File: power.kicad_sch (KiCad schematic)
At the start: 25 parts, among them U1 ECP5U_12_CABGA256, U2 TLV62569DBV, U3 TLV62569DBV, U4 TLV62569DBV

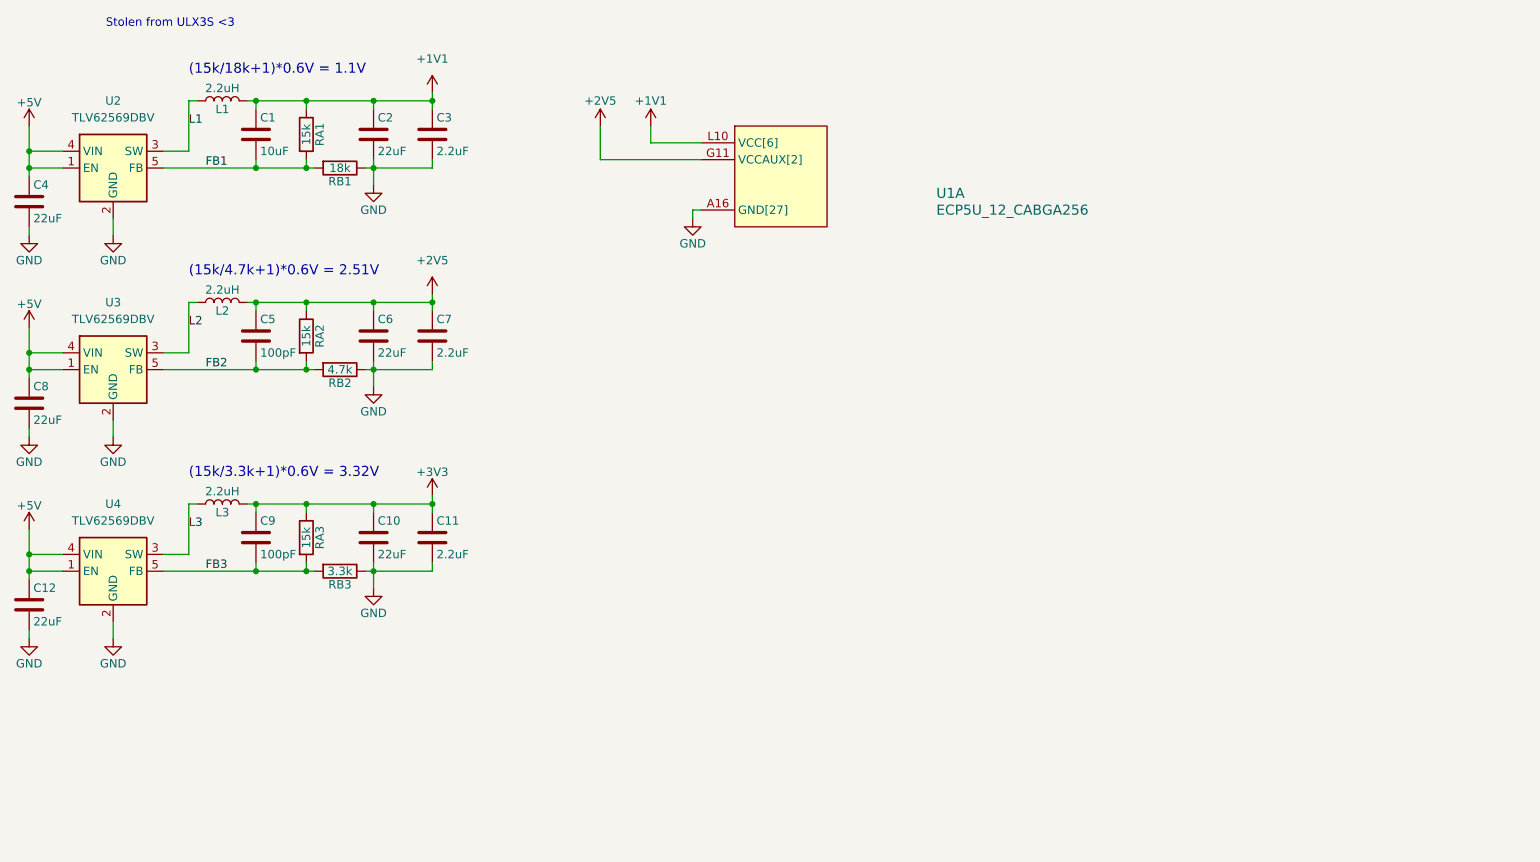
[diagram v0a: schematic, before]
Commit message: Stash
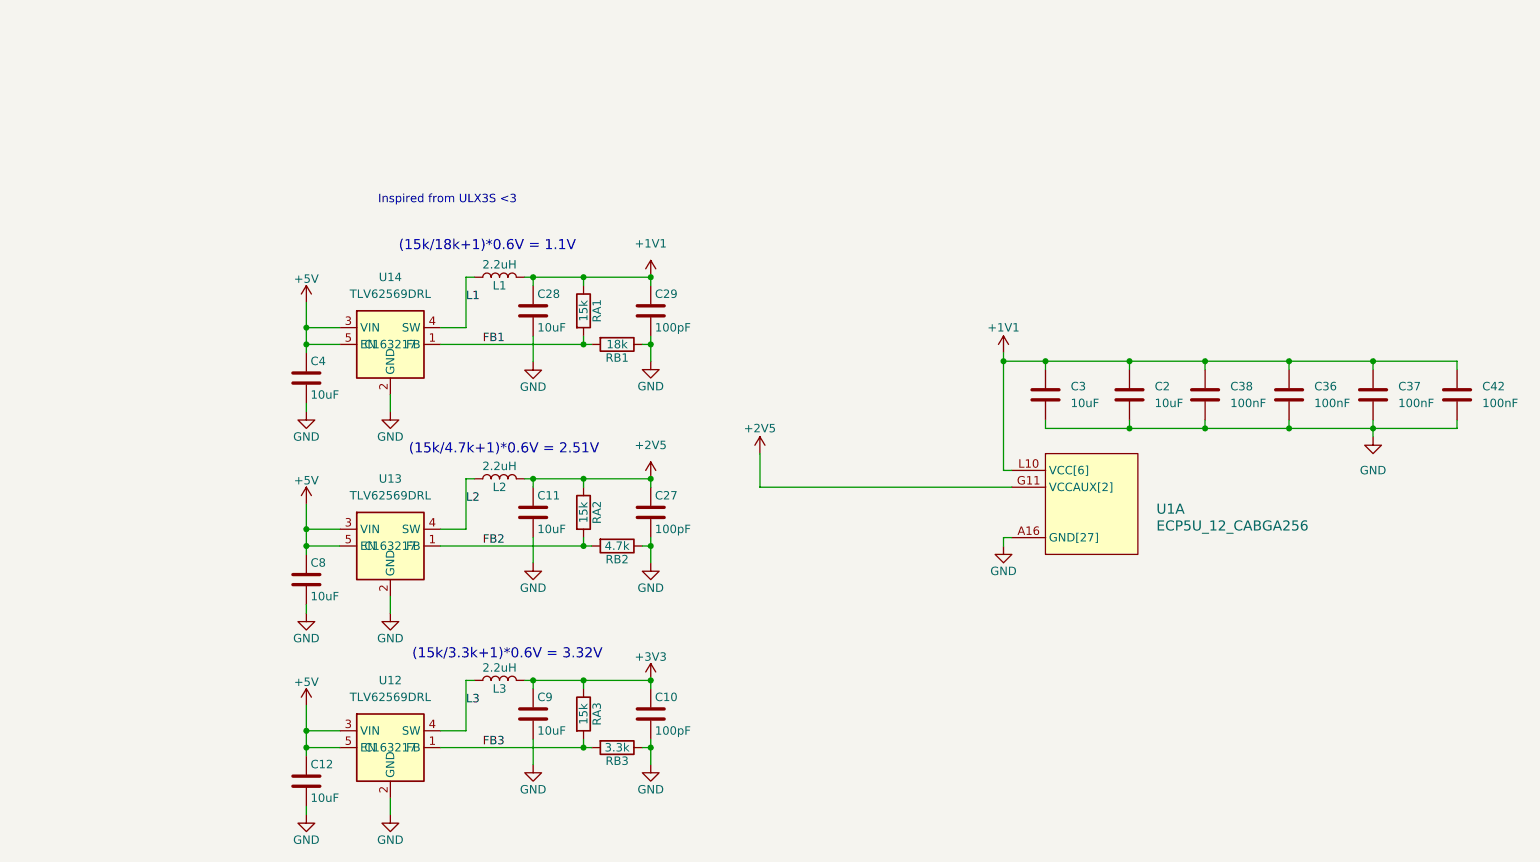
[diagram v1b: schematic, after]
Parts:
- removed C1: 10uF, Capacitor_SMD:C_0603_1608Metric, symbol Device:C
- removed C5: 100pF, Capacitor_SMD:C_0603_1608Metric, symbol Device:C
- removed C6: 22uF, Capacitor_SMD:C_0603_1608Metric, symbol Device:C
- removed C7: 2.2uF, Capacitor_SMD:C_0603_1608Metric, symbol Device:C
- removed U2, U3, U4: TLV62569DBV, Package_TO_SOT_SMD:SOT-23-5, symbol Regulator_Switching:TLV62569DBV
- added C27, C29: 100pF, Capacitor_SMD:C_0603_1608Metric, symbol Device:C
- added C28: 10uF, Capacitor_SMD:C_0603_1608Metric, symbol Device:C
- added C36, C37, C38, C42: 100nF, Capacitor_SMD:C_0402_1005Metric, symbol Device:C
- added U12, U13, U14: TLV62569DRL, Package_TO_SOT_SMD:SOT-563, symbol Regulator_Switching:TLV62569DRL
- C10: value 22uF -> 100pF
- C11, C3: value 2.2uF -> 10uF
- C12, C2, C4, C8: value 22uF -> 10uF
- C9: value 100pF -> 10uF
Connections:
- net +1V1: now also C28.1, C29.1, C36.1, C37.1, C38.1, C42.1
- net +2V5: now also C11.1, C27.1
- net +3V3: no longer C11.1
- net +5V: now also U12.3 (VIN), U12.5 (EN), U13.3 (VIN), U13.5 (EN), U14.3 (VIN), U14.5 (EN)
- net FB1: now also U14.1 (FB)
- net FB2: now also U13.1 (FB)
- net FB3: now also U12.1 (FB); no longer C9.2
- net GND: now also C9.2, C27.2, C28.2, C29.2, C36.2, C37.2, C38.2, C42.2, U12.2 (GND), U13.2 (GND), U14.2 (GND)
- net L1: now also U14.4 (SW)
- net L2: now also U13.4 (SW)
- net L3: now also U12.4 (SW)
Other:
- note added: "Inspired from ULX3S <3"
- note removed: "Stolen from ULX3S <3"
- moved on the sheet: C10, C12, C4, C8, C9, L1, L2, L3, RA1, RA2, RA3, RB1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
